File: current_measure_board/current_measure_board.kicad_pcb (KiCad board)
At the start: 6 copper layers, 76.2 x 76.2 mm, 39 parts, among them U1 LT6370HMS8-TRPBF, U2 LT1793AIS8-PBF, U3 LT1793AIS8-PBF, U4 LT1793AIS8-PBF

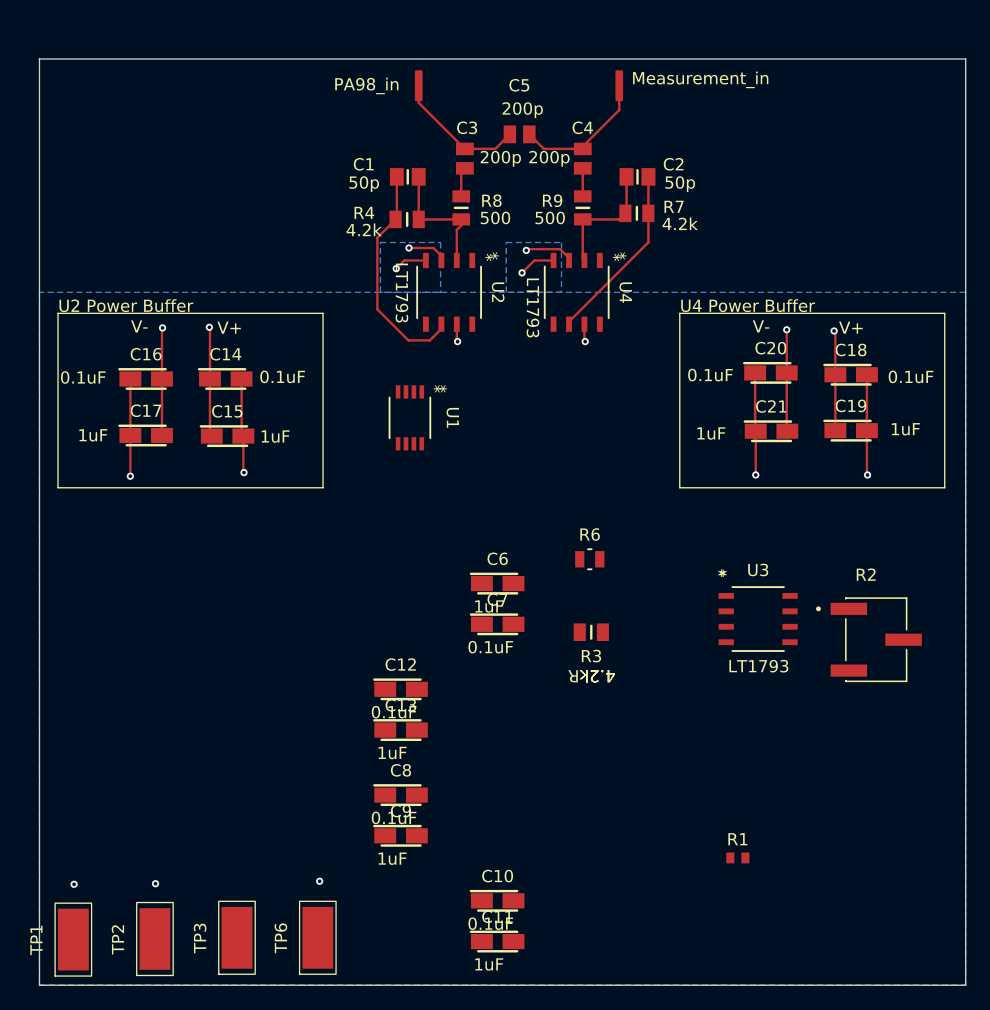
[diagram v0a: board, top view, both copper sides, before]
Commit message: Update
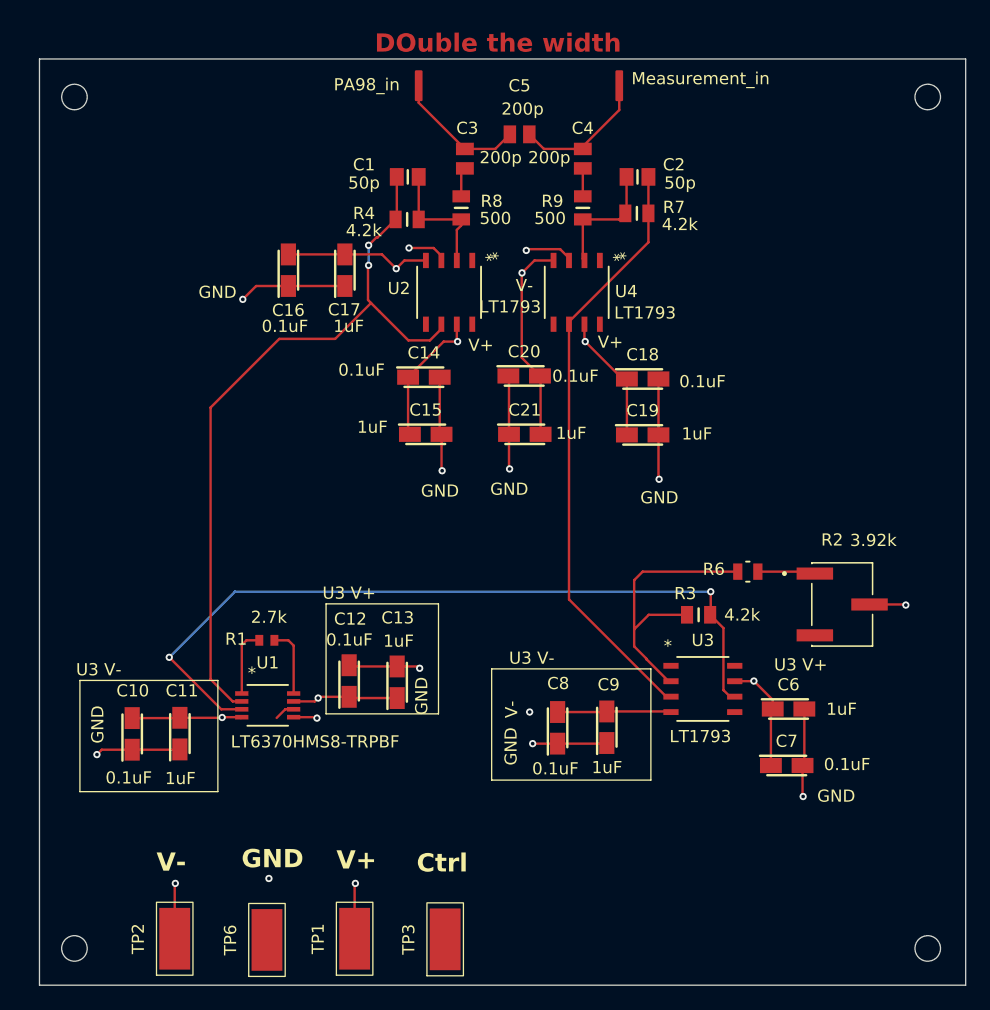
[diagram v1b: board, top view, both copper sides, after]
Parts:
- added REF**: MountingHole_2.1mm, MountingHole:MountingHole_2.1mm, F.Cu at (112.4, 60.9)
- added REF**: MountingHole_2.1mm, MountingHole:MountingHole_2.1mm, F.Cu at (182.6, 130.9)
- added REF**: MountingHole_2.1mm, MountingHole:MountingHole_2.1mm, F.Cu at (112.4, 130.9)
- added REF**: MountingHole_2.1mm, MountingHole:MountingHole_2.1mm, F.Cu at (182.6, 60.9)
- moved R1 42.7 mm to (128.2, 105.5)
- moved C10 33.1 mm to (117.2, 113.2), turned to 90 degrees
- moved C11 31.2 mm to (121.1, 113.2), turned to 90 degrees
- moved C7 26.5 mm to (171.0, 115.8)
- moved U1 26.4 mm to (128.3, 110.9), turned to 0 degrees
- moved C6 26.1 mm to (171.2, 111.2)
- moved TP1 23.1 mm to (137.9, 130.1)
- moved C17 21.3 mm to (134.7, 75.1), turned to 90 degrees
- moved C21 20.3 mm to (149.4, 88.6)
- moved C20 20.3 mm to (149.4, 83.8)
- moved C9 19.1 mm to (156.2, 112.7), turned to 90 degrees
- moved C18 17.2 mm to (159.2, 84.0)
- moved C19 17.2 mm to (159.2, 88.7)
- moved TP3 17.1 mm to (145.4, 130.2)
- moved C14 16.3 mm to (141.2, 83.9)
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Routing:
- net Net-(U1-IN+): track 0.00 -> 64.2 mm, vias 0 -> 2
- net Net-(U1-IN-): track 18.7 -> 61.8 mm, vias 0 -> 2
- net Net-(U3-+INA): track 14.8 -> 49.2 mm
- net GND: track 39.9 -> 71.5 mm, vias 7 -> 13
- net /Vminus: track 23.0 -> 52.4 mm
- net /Vplus: track 20.2 -> 45.0 mm
- net Net-(U3--INA): track 0.00 -> 23.4 mm
- net Net-(U1-RG+): track 0.00 -> 5.70 mm
- net Net-(U1-RG-): track 0.00 -> 5.59 mm
- net Net-(R2-Pad1): track 0.00 -> 4.75 mm
- net /Control_out: track 0.00 -> 1.69 mm
- added copper zone on In2.Cu, net GND
- removed copper zone on B.Cu, net GND
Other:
- board text added: "Ctrl"
- board text added: "DOuble the width"
- board text added: "GND"
- board text added: "U3 V+"
- board text added: "U3 V-"
- board text removed: "U2 Power Buffer"
- board text removed: "U4 Power Buffer"
